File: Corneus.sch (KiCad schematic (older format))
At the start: 146 parts

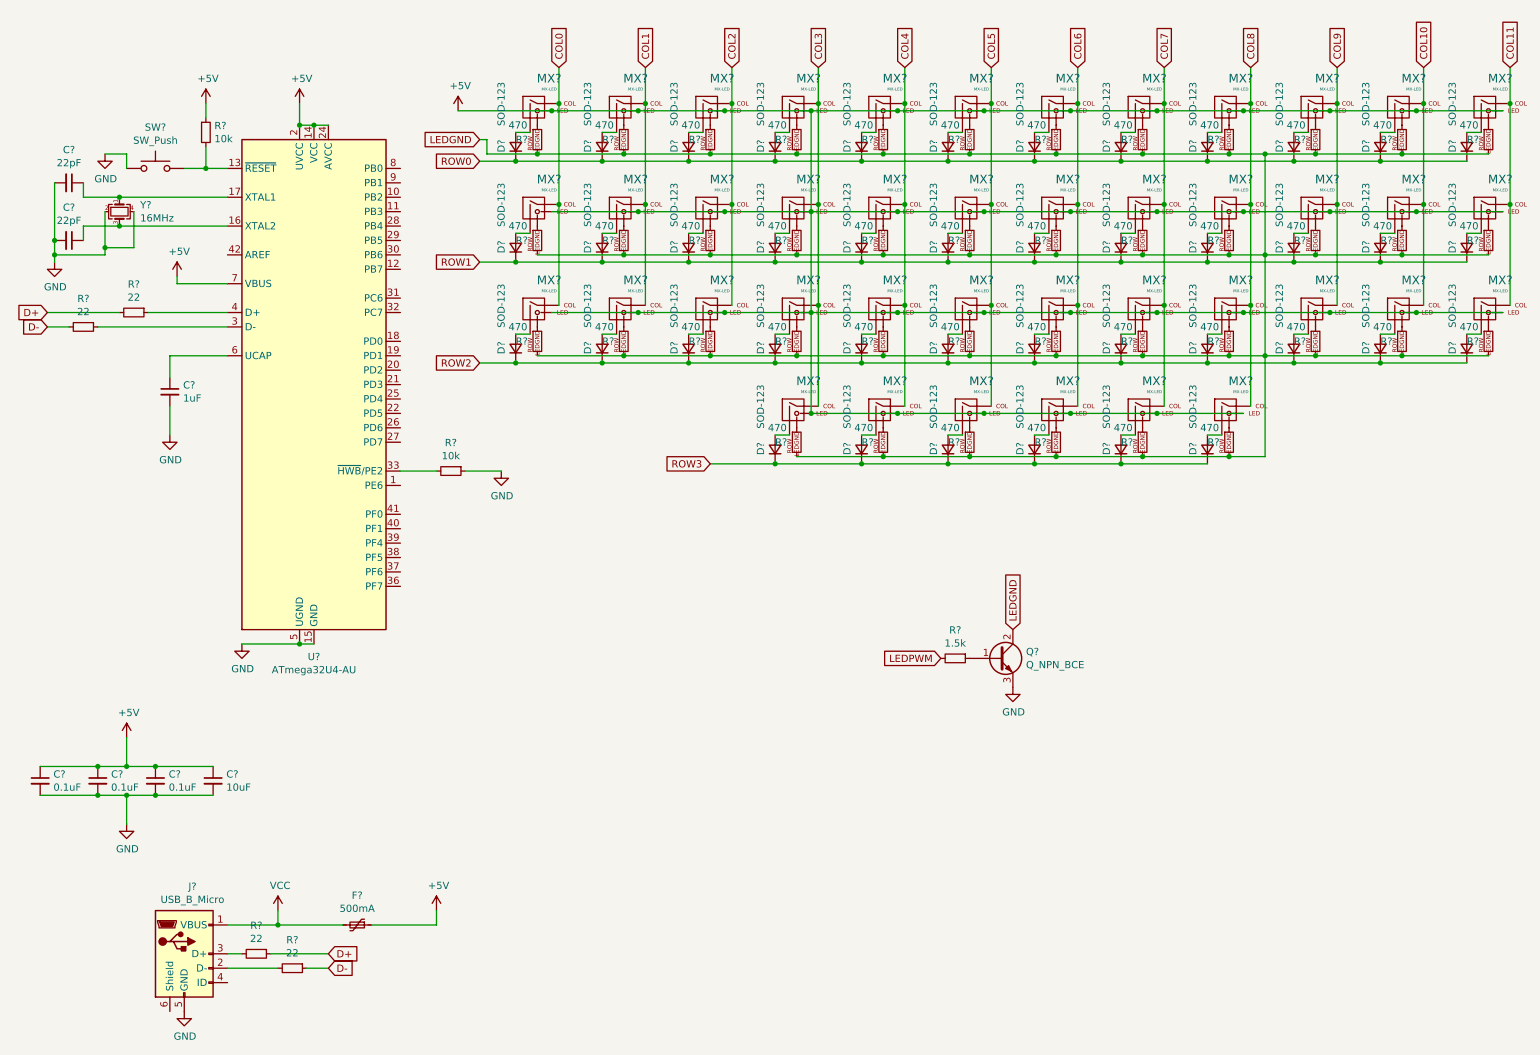
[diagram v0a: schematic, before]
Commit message: assigned reference designators
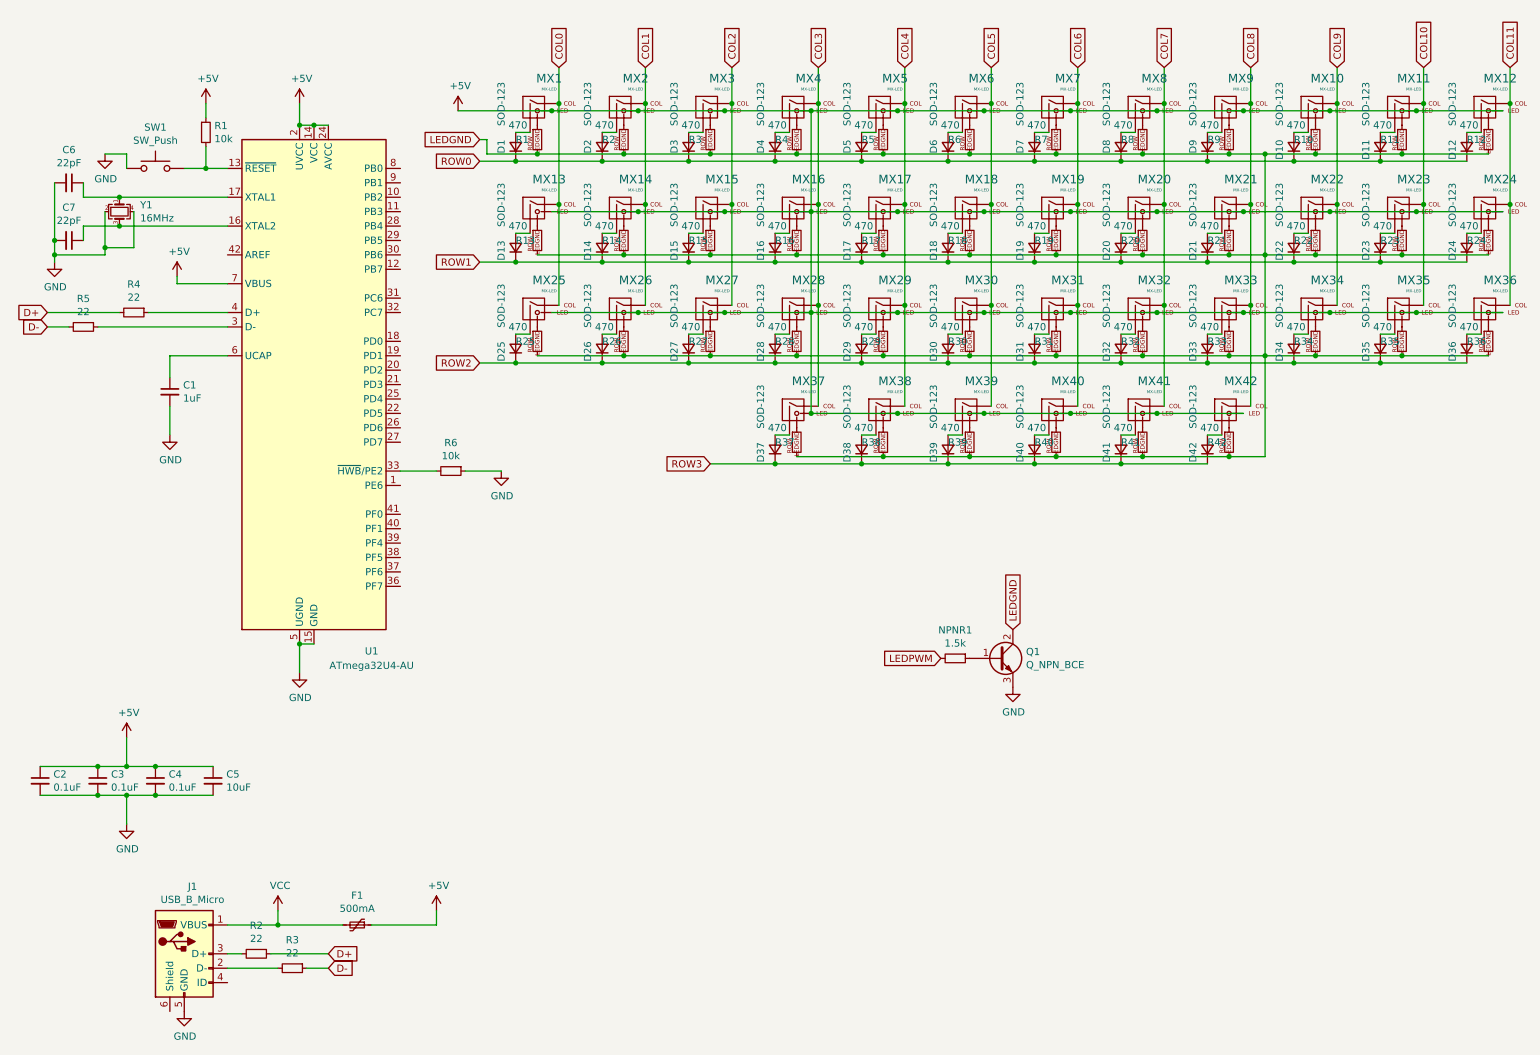
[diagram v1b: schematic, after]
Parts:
- gave numbers to parts that had none: 140
